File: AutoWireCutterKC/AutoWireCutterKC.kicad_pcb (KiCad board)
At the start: 2 copper layers, 17 parts, among them J1 LCD I/O, J2 ISP, J3 LCD Serial, J5 LCD Power, J6 Servo, J8 Barrel_Jack, J9 Stepper, U1 ATMEGA328P-AU, U2 MCP1700_SOT23, U3 LT1129-5.0_SOT223

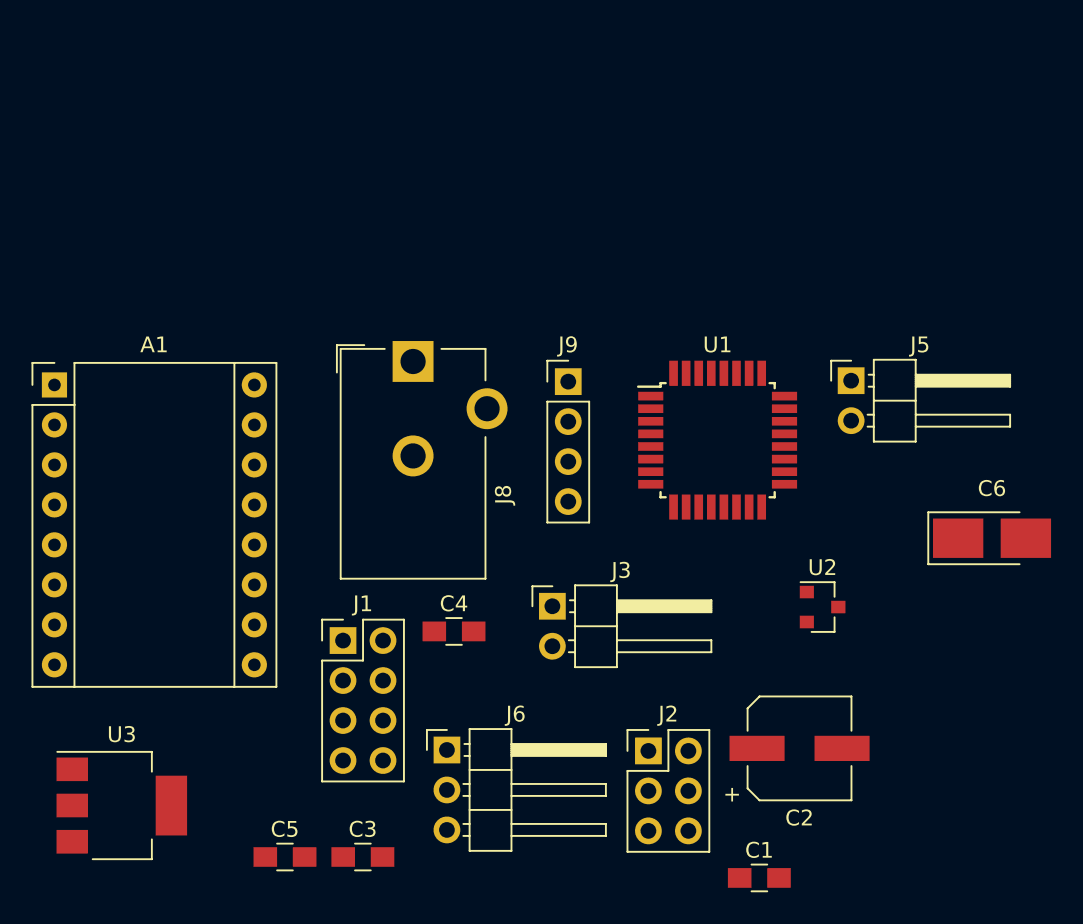
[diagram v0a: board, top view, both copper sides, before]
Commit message: PCB Populated
Traces needed
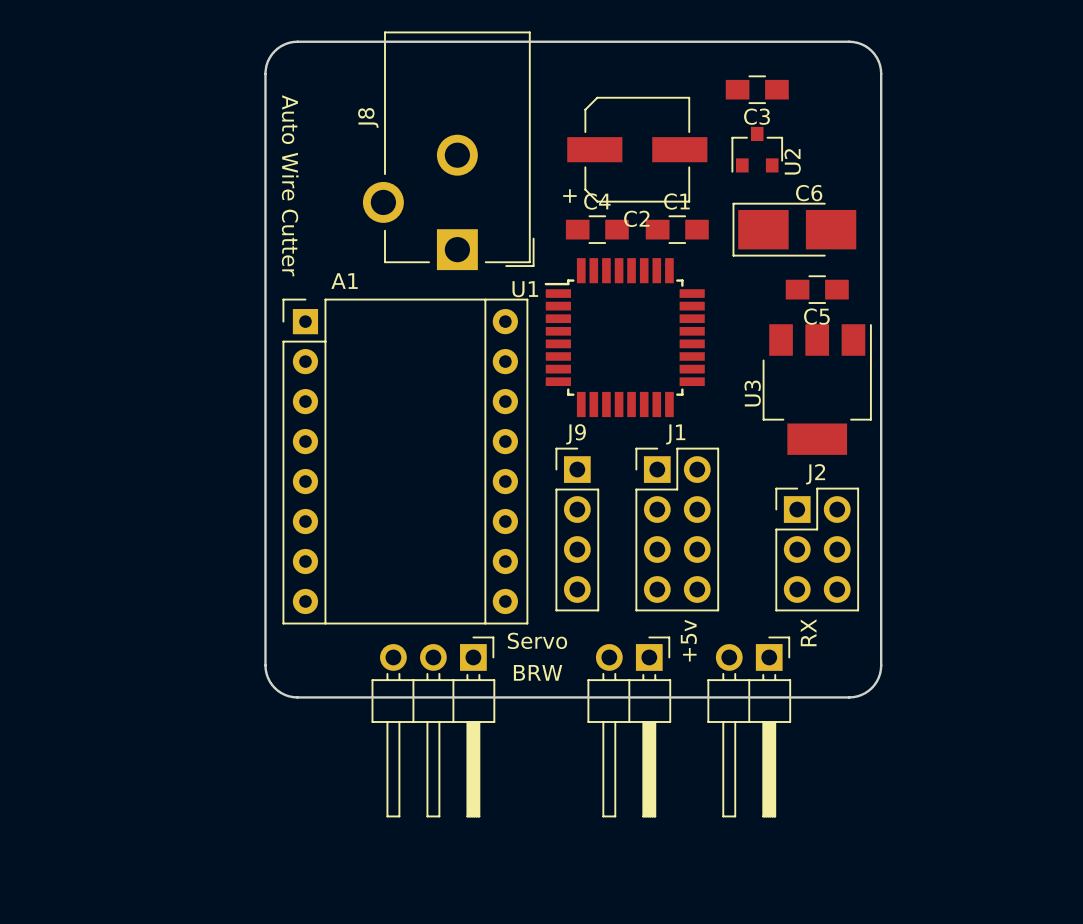
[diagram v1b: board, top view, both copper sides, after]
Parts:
- removed J3: LCD Serial, Pin_Headers:Pin_Header_Angled_1x02_Pitch2.54mm
- removed J5: LCD Power, Pin_Headers:Pin_Header_Angled_1x02_Pitch2.54mm
- removed J6: Servo, Pin_Headers:Pin_Header_Angled_1x03_Pitch2.54mm
- added +5v: LCD Power, Pin_Headers:Pin_Header_Angled_1x02_Pitch2.54mm, F.Cu at (159.5, 117.3)
- added RX: LCD Serial, Pin_Headers:Pin_Header_Angled_1x02_Pitch2.54mm, F.Cu at (167.1, 117.3)
- added Servo: Servo, Pin_Headers:Pin_Header_Angled_1x03_Pitch2.54mm, F.Cu at (148.3, 117.3)
- moved C3 54.8 mm to (166.4, 81.3), turned to 180 degrees
- moved U3 51.5 mm to (170.2, 100.3), turned to 270 degrees
- moved C5 49.4 mm to (170.2, 94.0), turned to 180 degrees
- moved C1 41.5 mm to (161.3, 90.2)
- moved C2 39.4 mm to (158.8, 85.1)
- moved U2 29.3 mm to (166.4, 85.1), turned to 90 degrees
- moved C4 27.1 mm to (156.2, 90.2)
- moved C6 23.2 mm to (168.9, 90.2)
- moved J1 22.7 mm to (160.0, 105.4)
- moved J2 18.0 mm to (168.9, 108.0)
- moved A1 16.4 mm to (137.7, 96.0)
- moved U1 8.77 mm to (158.0, 97.0)
- moved J8 7.64 mm to (147.3, 91.4), turned to 180 degrees
- moved J9 5.61 mm to (154.9, 105.4)
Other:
- board outline added: 39.1 x 41.7 mm
- board text added: "Auto Wire Cutter"
- board text added: "BRW"
